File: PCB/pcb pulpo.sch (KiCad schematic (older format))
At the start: 48 parts, among them J1 fan1, J10 fan8, J11 fan8, J12 izq, J13 dcha, J2 Entrada 12V, J3 fan2, J4 fan3, J5 fan4, J6 fan5, J7 fan6, J8 fan7, J9 fan8, Q1 IRF540N, Q10 IRF540N, Q2 IRF540N, Q3 IRF540N, Q4 IRF540N, Q5 IRF540N, Q6 IRF540N, Q7 IRF540N, Q8 IRF540N, Q9 IRF540N, U1 Teensy3.0, U2 LM7805_TO220

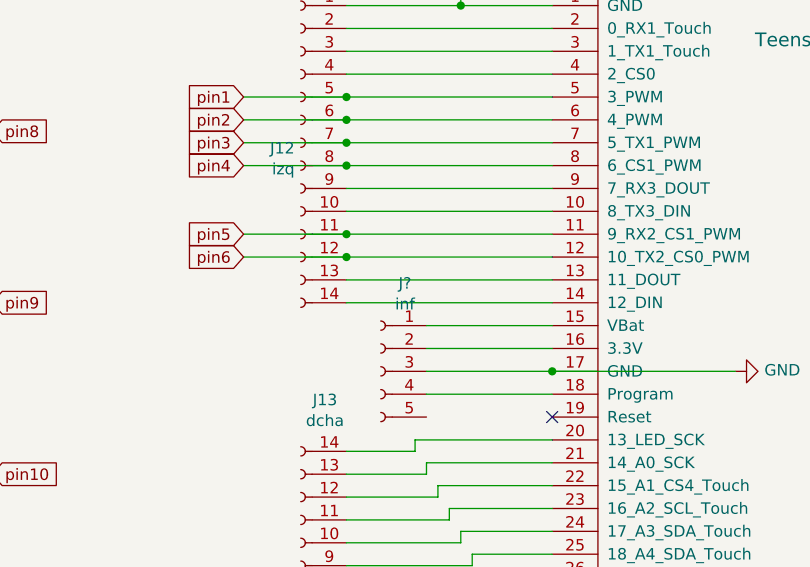
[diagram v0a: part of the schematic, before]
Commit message: Boceto PCB
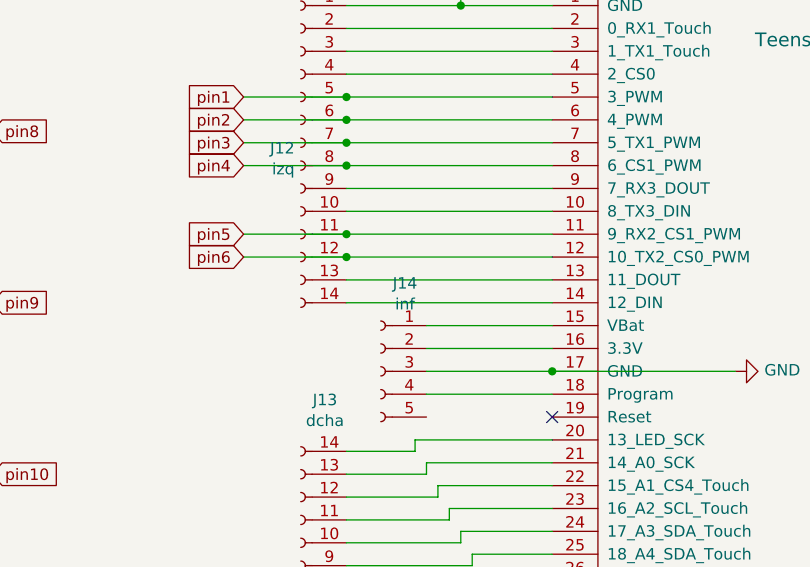
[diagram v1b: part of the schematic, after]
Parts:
- J12, J13: footprint (none) -> Connector_PinSocket_2.54mm:PinSocket_1x14_P2.54mm_Vertical
- J14: renamed from J?; footprint (none) -> Connector_PinSocket_2.54mm:PinSocket_1x05_P2.54mm_Vertical
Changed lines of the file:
@@
 F 0 "J12" H 5677 2826 50  0000 L CNN
 F 1 "izq" H 5677 2735 50  0000 L CNN
-F 2 "" H 5650 2850 50  0001 C CNN
+F 2 "Connector_PinSocket_2.54mm:PinSocket_1x14_P2.54mm_Vertical" H 5650 2850 50  0001 C CNN
 F 3 "~" H 5650 2850 50  0001 C CNN
 	1    5650 2850
@@
 F 0 "J13" H 5544 3975 50  0000 C CNN
 F 1 "dcha" H 5544 4066 50  0000 C CNN
-F 2 "" H 5650 4900 50  0001 C CNN
+F 2 "Connector_PinSocket_2.54mm:PinSocket_1x14_P2.54mm_Vertical" H 5650 4900 50  0001 C CNN
 F 3 "~" H 5650 4900 50  0001 C CNN
 	1    5650 4900
@@
 	9350 3550 8950 3550
 $Comp
-L Connector:Conn_01x05_Female J?
+L Connector:Conn_01x05_Female J14
 U 1 1 5C2E0A99
 P 6000 3850
-F 0 "J?" H 5894 4235 50  0000 C CNN
+F 0 "J14" H 5894 4235 50  0000 C CNN
 F 1 "inf" H 5894 4144 50  0000 C CNN
-F 2 "" H 6000 3850 50  0001 C CNN
+F 2 "Connector_PinSocket_2.54mm:PinSocket_1x05_P2.54mm_Vertical" H 6000 3850 50  0001 C CNN
 F 3 "~" H 6000 3850 50  0001 C CNN
 	1    6000 3850
